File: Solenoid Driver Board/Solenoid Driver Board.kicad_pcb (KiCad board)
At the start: 2 copper layers, 33 parts, among them J1 AIN2, J10 DEBUG, J2 CH1, J3 CH2, J4 CH3, J5 BUS-O, J6 BUS-I, J7 RGB_LED, J8 Solenoid, J9 I2C, Q1 IRLB8721PBF, U1 AMS1117-5.0, U2 STM8S003F3P

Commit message: New source image
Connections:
- D1 pad 2: CH1 -> CH0
- D2 pad 2: CH2 -> CH1
- D3 pad 2: CH3 -> CH2
- J2 pad 1: CH1 -> CH0
- J3 pad 1: CH2 -> CH1
- J4 pad 1: CH3 -> CH2
- U2 pad 10: CH1 -> CH0
- U2 pad 15: CH2 -> CH1
- U2 pad 20: CH3 -> CH2

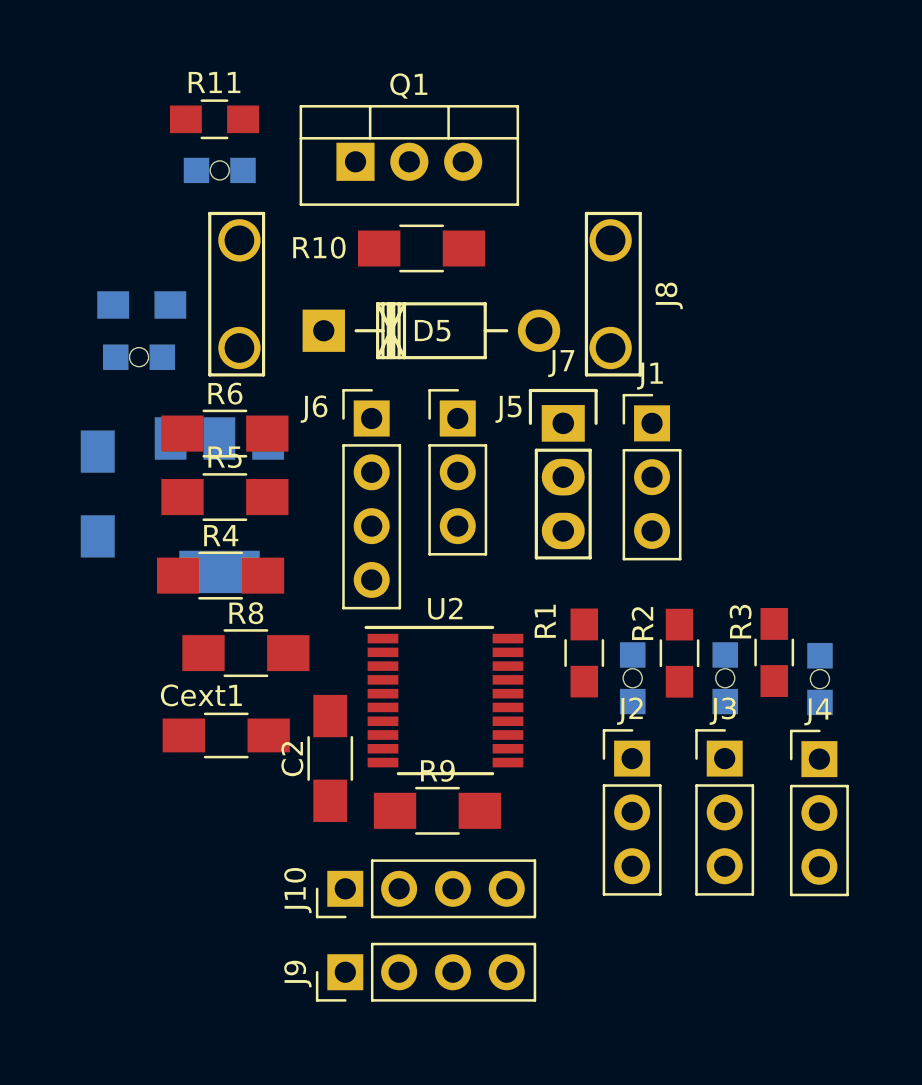
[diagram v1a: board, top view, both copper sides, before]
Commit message: PWM Test, lots of work on v1.1 PCBs
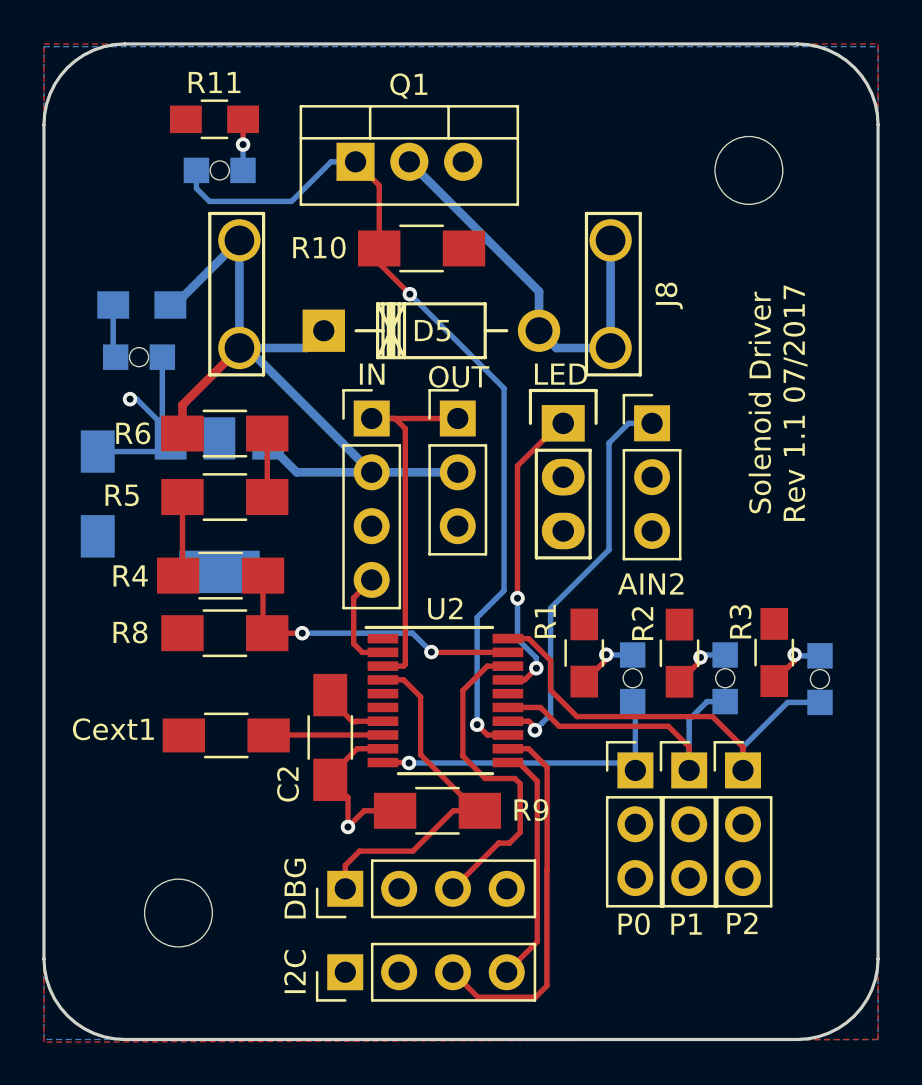
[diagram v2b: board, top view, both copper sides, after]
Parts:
- added REF**: MountingHole_3.2mm_M3, Mounting_Holes:MountingHole_3.2mm_M3, F.Cu at (229.4, 85.5)
- added REF**: MountingHole_3.2mm_M3, Mounting_Holes:MountingHole_3.2mm_M3, F.Cu at (202.4, 120.5)
- moved P2 3.65 mm to (229.1, 113.8)
- moved P1 1.77 mm to (226.5, 113.8)
- moved R8 1.37 mm to (204.6, 107.3)
- moved C2 0.99 mm to (209.6, 112.2)
- moved P0 0.58 mm to (224.0, 113.8)
- renumbered J1 to AIN2, J10 to DBG, J9 to I2C, J6 to IN, J7 to LED, J5 to OUT, J2 to P0, J3 to P1, J4 to P2
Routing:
- net PC3: track 0.00 -> 41.0 mm, vias 0 -> 2
- net +12V: track 0.00 -> 37.5 mm
- net CH2: track 0.00 -> 20.8 mm
- net Net-(D5-Pad2): track 0.00 -> 19.3 mm
- net AIN2: track 0.00 -> 18.9 mm, vias 0 -> 1
- net RX: track 0.00 -> 18.1 mm
- net SCL: track 0.00 -> 17.7 mm
- net NRST: track 0.00 -> 17.3 mm
- net CH0: track 0.00 -> 16.2 mm, vias 0 -> 1
- net SWIM: track 0.00 -> 15.5 mm
- net CH1: track 0.00 -> 14.9 mm
- net VIN_A: track 0.00 -> 14.5 mm, vias 0 -> 2
- net Net-(J7-Pad1): track 0.00 -> 14.5 mm, vias 0 -> 2
- net GND: track 0.00 -> 13.7 mm, vias 0 -> 1
- net SDA: track 0.00 -> 11.4 mm
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- added copper zone on B.Cu, net +5V
- added copper zone on F.Cu, net GND
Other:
- board outline added: 39.4 x 47 mm
- board text added: "Solenoid Driver Rev 1.1 07/2017"
